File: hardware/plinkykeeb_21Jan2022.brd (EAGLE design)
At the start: 254 x 43.2 mm, 94 parts, among them J1 SJ-3523-SMT, J2 SJ-3523-SMT, SW1 KAILH_SOCKETBOX_JADE, SW10 KAILH_SOCKETBOX_JADE, SW11 KAILH_SOCKETBOX_JADE, SW12 KAILH_SOCKETBOX_JADE, SW13 KAILH_SOCKETBOX_JADE, SW14 KAILH_SOCKETBOX_JADE, SW15 KAILH_SOCKETBOX_JADE, SW16 KAILH_SOCKETBOX_JADE, SW17 KAILH_SOCKETBOX_JADE, SW18 KAILH_SOCKETBOX_JADE, SW19 KAILH_SOCKETBOX_JADE, SW2 KAILH_SOCKETBOX_JADE, SW20 KAILH_SOCKETBOX_JADE, SW3 KAILH_SOCKETBOX_JADE, SW4 KAILH_SOCKETBOX_JADE, SW5 KAILH_SOCKETBOX_JADE, SW6 KAILH_SOCKETBOX_JADE, SW7 KAILH_SOCKETBOX_JADE, SW8 KAILH_SOCKETBOX_JADE, SW9 KAILH_SOCKETBOX_JADE, U1 PRO_MICRO

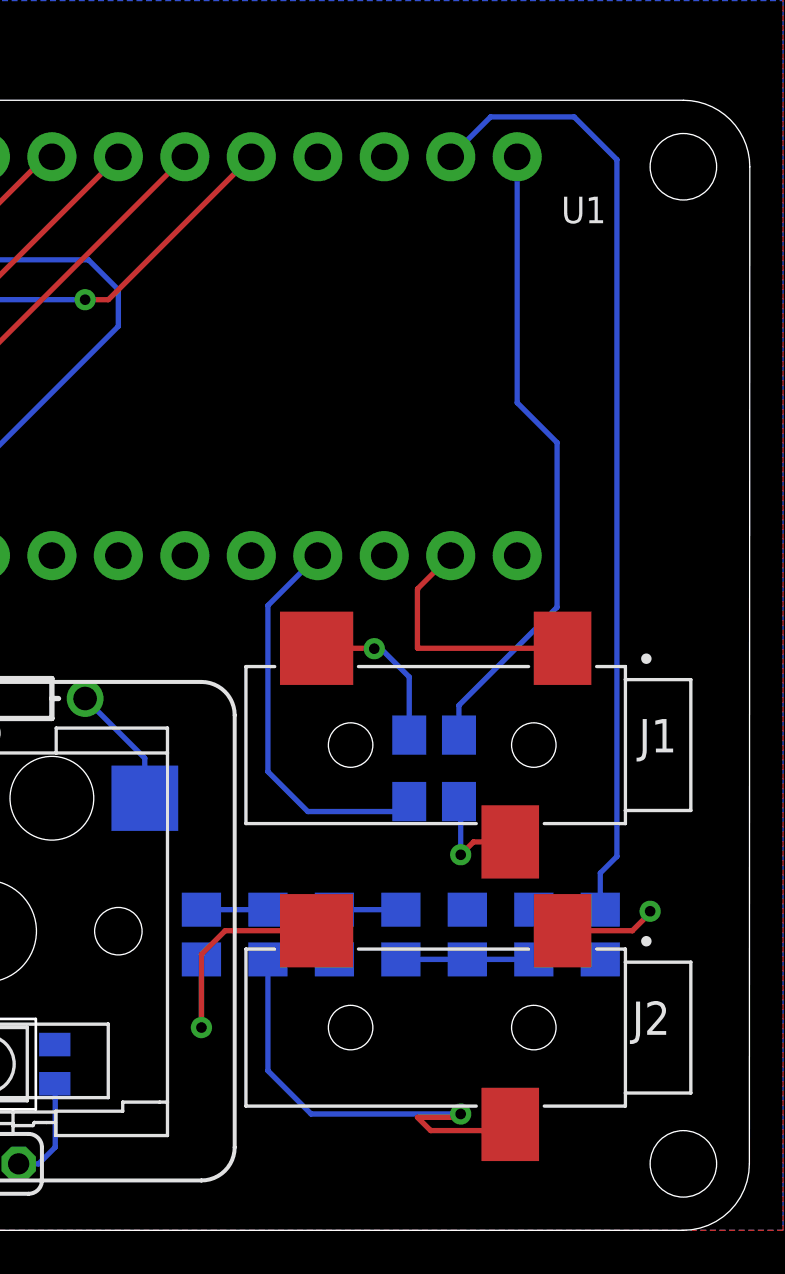
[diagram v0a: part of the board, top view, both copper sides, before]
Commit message: docs
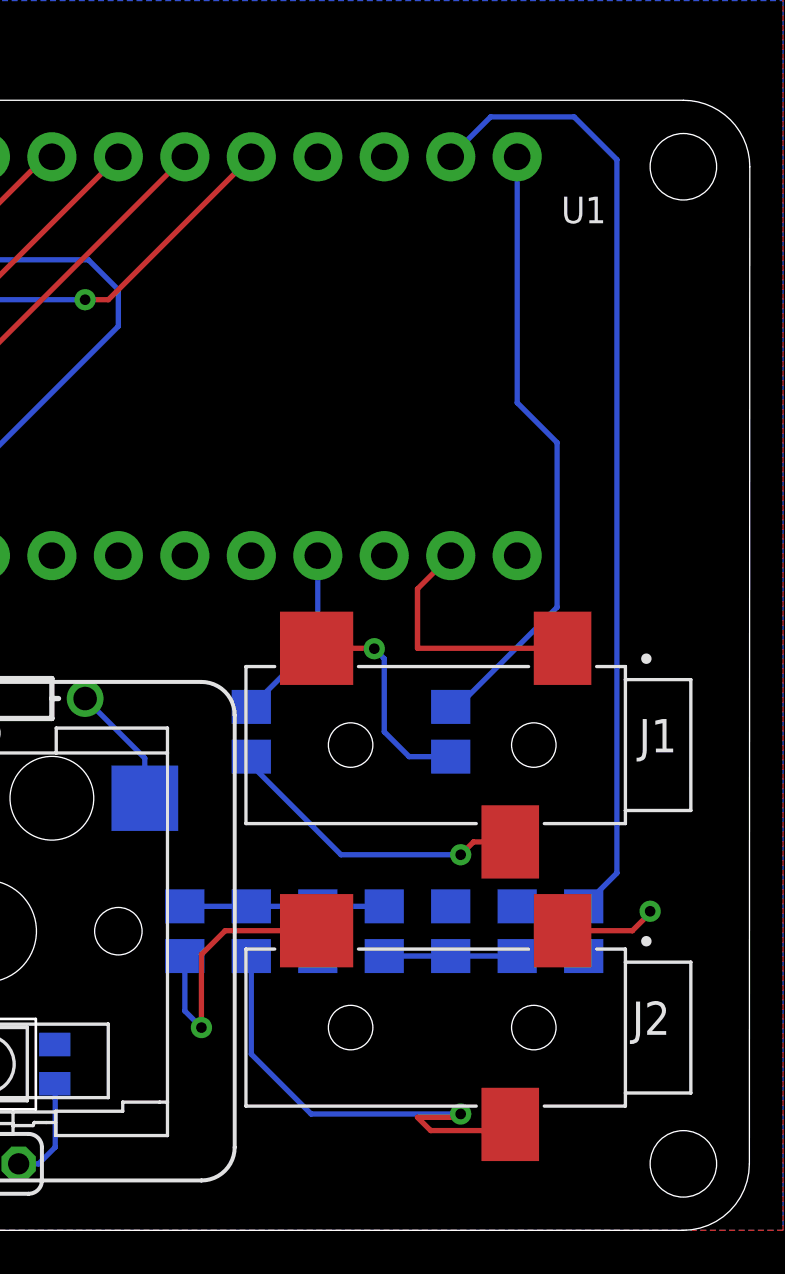
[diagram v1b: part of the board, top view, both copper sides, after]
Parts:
- moved R2 7.48 mm to (234.9, 19.1), turned to 90 degrees
- moved C22 0.65 mm to (242.6, 11.4)
- moved R4 0.65 mm to (234.9, 11.4)
- moved R1 0.65 mm to (242.6, 19.1), turned to 90 degrees
- moved C21 0.65 mm to (240.0, 11.4)
- moved R3 0.65 mm to (232.4, 11.4)
- moved R5 0.65 mm to (237.5, 11.4)
- moved R6 0.65 mm to (245.1, 11.4)
- moved R7 0.65 mm to (247.7, 11.4)
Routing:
- net +3V3: track 15.2 -> 6.83 mm
- net N$43: track 4.16 -> 11.8 mm
- net N$42: track 6.22 -> 8.48 mm
- net MIDIOUT: track 24.3 -> 23.5 mm
